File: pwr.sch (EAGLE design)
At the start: 44 parts, among them Q1 IPD65R600C6, T1 750811647, U1 UCC28700, U3 ESP-WROOM-32

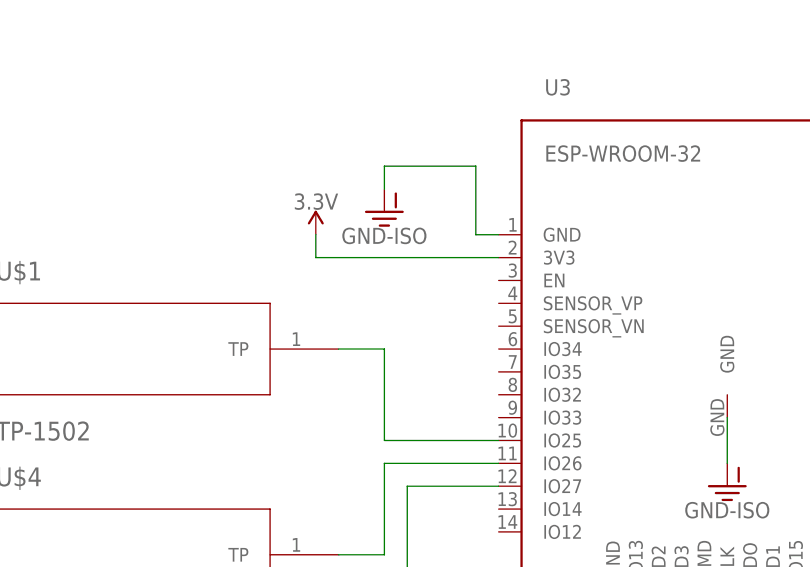
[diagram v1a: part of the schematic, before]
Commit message: ordered
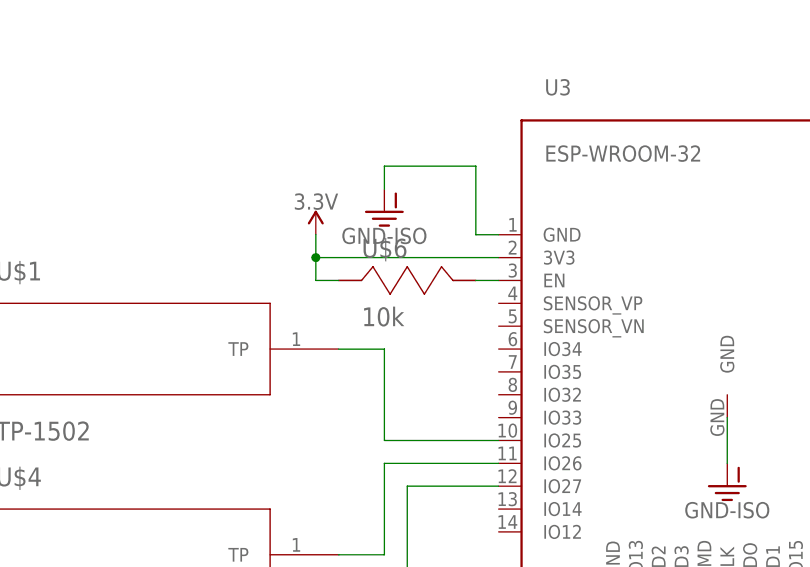
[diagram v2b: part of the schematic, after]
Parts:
- added U$6: 10k, derek:CRCW060310K0FKEA
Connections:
- new net N$22: U$6.1, U3.EN
- net 3.3V: now also U$6.2
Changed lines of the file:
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@@
 <part name="GND-ISO8" library="derek" deviceset="GND-ISO" device=""/>
 <part name="U$5" library="derek" deviceset="TP-1502" device=""/>
+<part name="U$6" library="derek" deviceset="CRCW060310K0FKEA" device="" value="10k"/>
 </parts>
 <sheets>
@@
 <instance part="GND-ISO8" gate="G$1" x="472.44" y="-68.58"/>
 <instance part="U$5" gate="A" x="429.26" y="-96.52"/>
+<instance part="U$6" gate="G$1" x="436.88" y="-45.72"/>
 </instances>
 <busses>
@@
 <wire x1="447.04" y1="-43.18" x2="426.72" y2="-43.18" width="0.1524" layer="91"/>
 <wire x1="426.72" y1="-43.18" x2="426.72" y2="-40.64" width="0.1524" layer="91"/>
+<pinref part="U$6" gate="G$1" pin="2"/>
+<wire x1="429.26" y1="-45.72" x2="426.72" y2="-45.72" width="0.1524" layer="91"/>
+<wire x1="426.72" y1="-45.72" x2="426.72" y2="-43.18" width="0.1524" layer="91"/>
+<junction x="426.72" y="-43.18"/>
 </segment>
 </net>
@@
 </segment>
 </net>
+<net name="N$22" class="0">
+<segment>
+<pinref part="U$6" gate="G$1" pin="1"/>
+<pinref part="U3" gate="G$1" pin="EN"/>
+<wire x1="444.5" y1="-45.72" x2="447.04" y2="-45.72" width="0.1524" layer="91"/>
+</segment>
+</net>
